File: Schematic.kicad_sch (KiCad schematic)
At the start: 73 parts, among them J1 Screw_Terminal_01x04, J20 T44007, J21 T44007, Q1 HY1707, Q20 2N2222, Q21 PMOS, U1 UC3845, U20 SFH618A-5, U21 TL431LP, U23 TCMT1108, U24 UC3843_SOIC8, U26 TL432DBZ

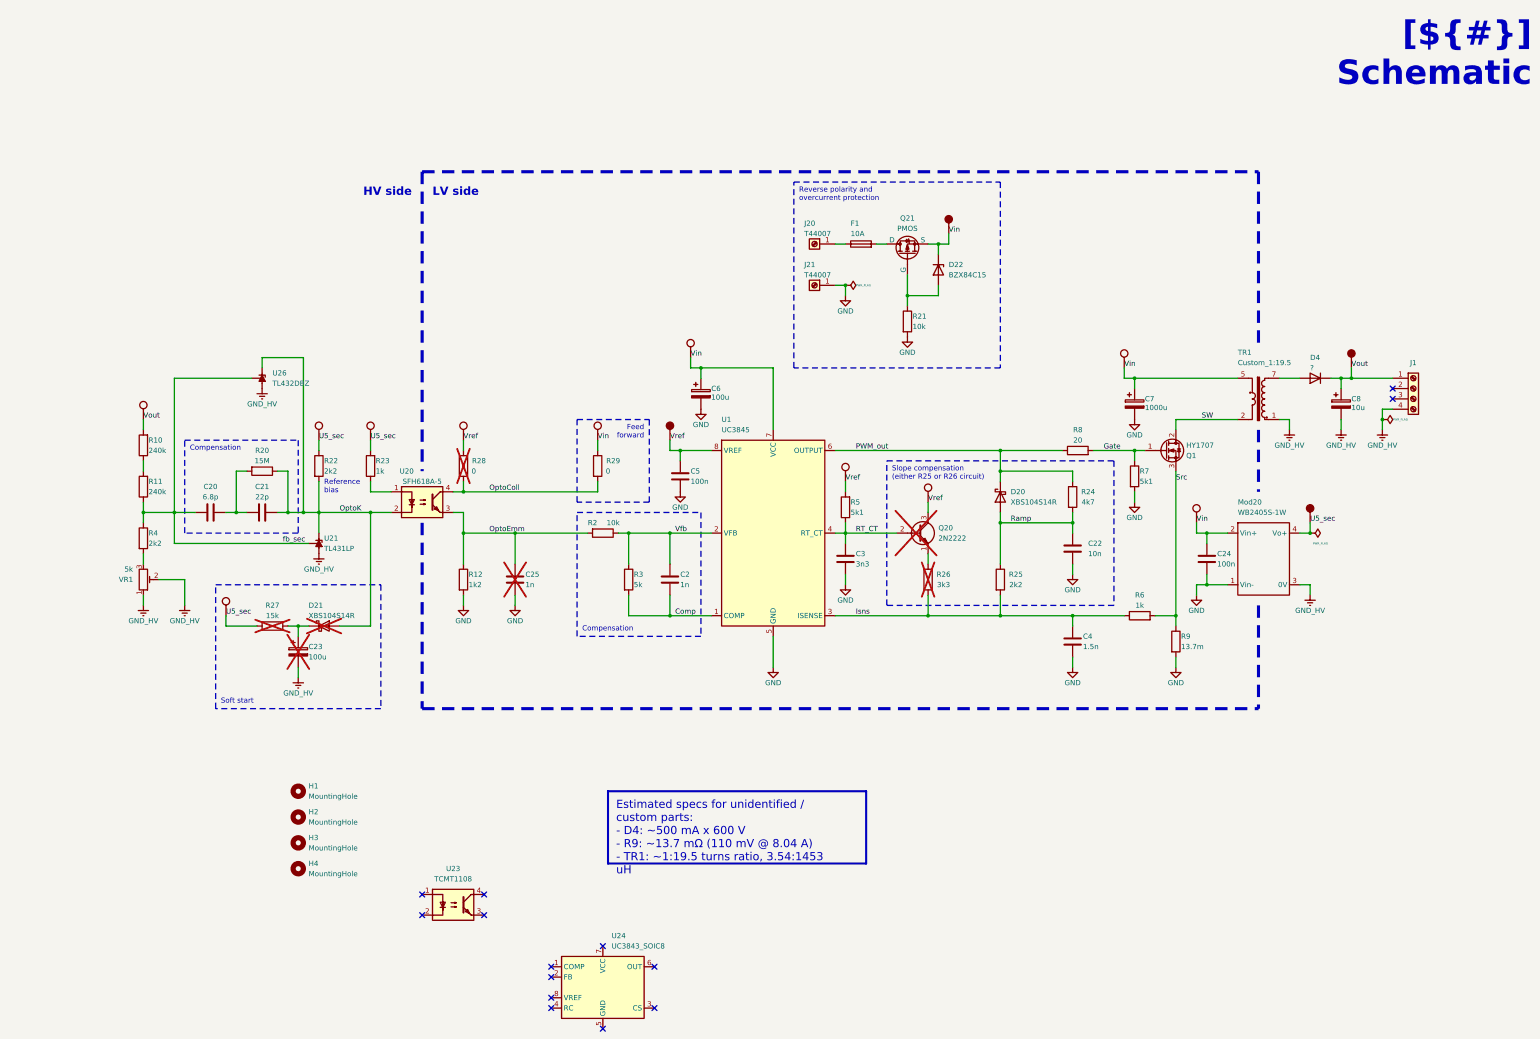
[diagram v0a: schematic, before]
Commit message: Several footprint updates
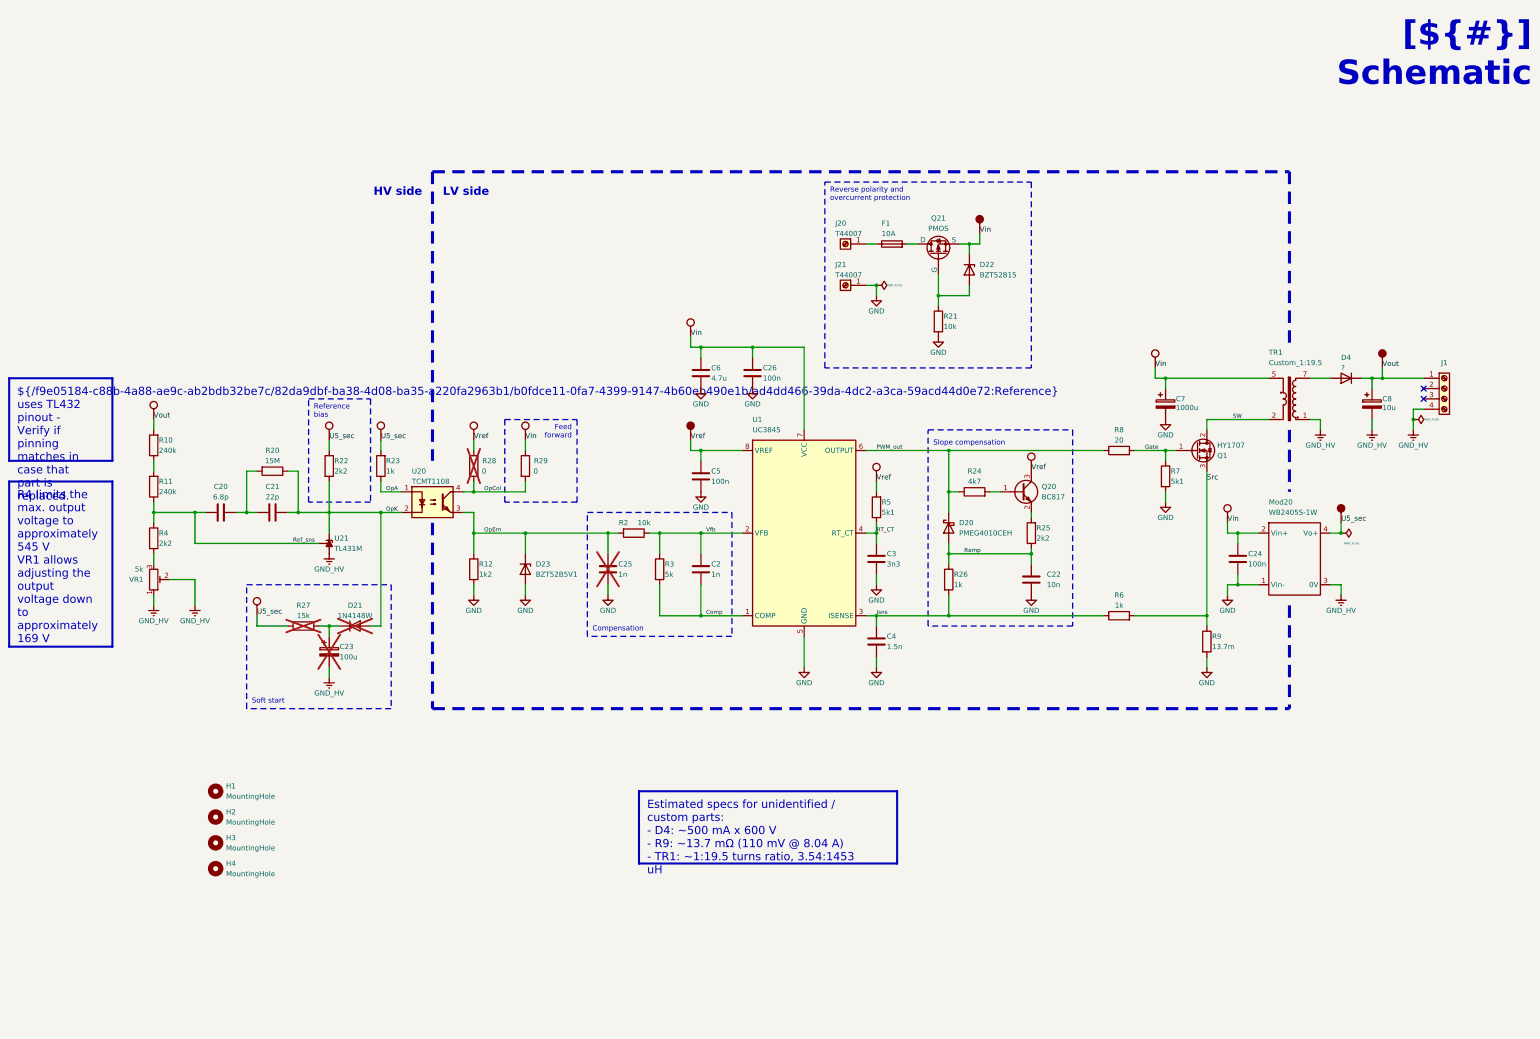
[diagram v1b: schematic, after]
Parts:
- removed C6: 100u, Capacitor_THT:C_Radial_D8.0mm_H11.5mm_P3.50mm, symbol Device:C_Polarized
- removed Q20: 2N2222, Package_TO_SOT_THT:TO-92L_Inline_Wide, symbol Transistor_BJT:2N3904
- removed U20: SFH618A-5, Package_DIP:DIP-4_W7.62mm, symbol Isolator:SFH617A-1
- removed U21: TL431LP, Package_TO_SOT_THT:TO-92L_Inline_Wide, symbol Reference_Voltage:TL431LP
- removed U24: UC3843_SOIC8, Package_SO:SOIC-8_3.9x4.9mm_P1.27mm, symbol Regulator_Controller:UC3843_SOIC8
- added C26: 100n, Capacitor_SMD:C_0603_1608Metric_Pad1.08x0.95mm_HandSolder, symbol Device:C
- added C6: 4.7u, Capacitor_SMD:C_0805_2012Metric_Pad1.18x1.45mm_HandSolder, symbol Device:C
- added D23: BZT52B5V1, Diode_SMD:D_SOD-123, symbol Device:D_Zener
- added Q20: BC817, Package_TO_SOT_SMD:SOT-23, symbol Transistor_BJT:BC817
- D20: value XBS104S14R -> PMEG4010CEH; symbol Device:D_Schottky -> Diode:PMEG4010CEH
- D21: value XBS104S14R -> 1N4148W; footprint Diode_SMD:D_SOD-123F -> Diode_SMD:D_SOD-123; symbol Device:D_Schottky -> Diode:1N4148W
- D22: value BZX84C15 -> BZT52B15; footprint Package_TO_SOT_SMD:SOT-23 -> Diode_SMD:D_SOD-123; symbol Diode:BZX84Cxx -> Diode:BZT52Bxx
- F1: footprint Fuse:Fuseholder_Clip-5x20mm_Eaton_1A5601-01_Inline_P20.80x6.76mm_D1.70mm_Horizontal -> Fuse:Fuseholder_Clip-5x20mm_Littelfuse_520_Inline_P20.50x5.80mm_D1.30mm_Horizontal
- R26: value 3k3 -> 1k; now fitted
- U1: footprint Package_DIP:DIP-8_W7.62mm -> Package_SO:JEITA_SOIC-8_3.9x4.9mm_P1.27mm
- U21: renamed from U26; value TL432DBZ -> TL431M; Link (none) -> https://www.lcsc.com/product-detail/C48947167.html; MPN (none) -> FOSAN TL431M-0.3%-6AF
- renumbered U23 to U20
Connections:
- net OptoColl is gone; now on net OpCol: R28.2, R29.2
- net OptoEmm is gone; now on net OpEm: C25.1, R12.1, R2.2
- net OptoK is gone; now on net OpK: C21.2, D21.2 (A), R20.1, R22.2, U21.2 (K)
- net GND: now also C26.2, C6.2, D23.2 (A)
- net Isns: no longer R25.2
- net Ramp: now also R26.1; no longer R24.2
- net Vin: now also D22.1 (K), C26.1, C6.1; no longer D22.3 (K)
- net Vref: now also Q20.3 (C)
- net at Q21.2 (G), R21.1: now also D22.2 (A); no longer D22.1 (A)
- net OpA: now reaches U20.1
- net OpA: now also R23.1
- net OpK: now reaches U20.2
- net OpEm: now reaches U20.3
- net OpEm: now also D23.1 (K)
- net OpCol: now reaches U20.4
- net fb_sec renamed Ref_sns
- new net: Q20.1 (B), R24.2
- new net: Q20.2 (E), R25.2
- no-connect marks 14 -> 2
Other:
- note added: "Slope compensation"
- note removed: "Slope compensation (either R25 or R26 circuit)"
- moved on the sheet: C2, C20, C21, C22, C23, C24, C25, C3, C4, C5, C7, C8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

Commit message: Layout started
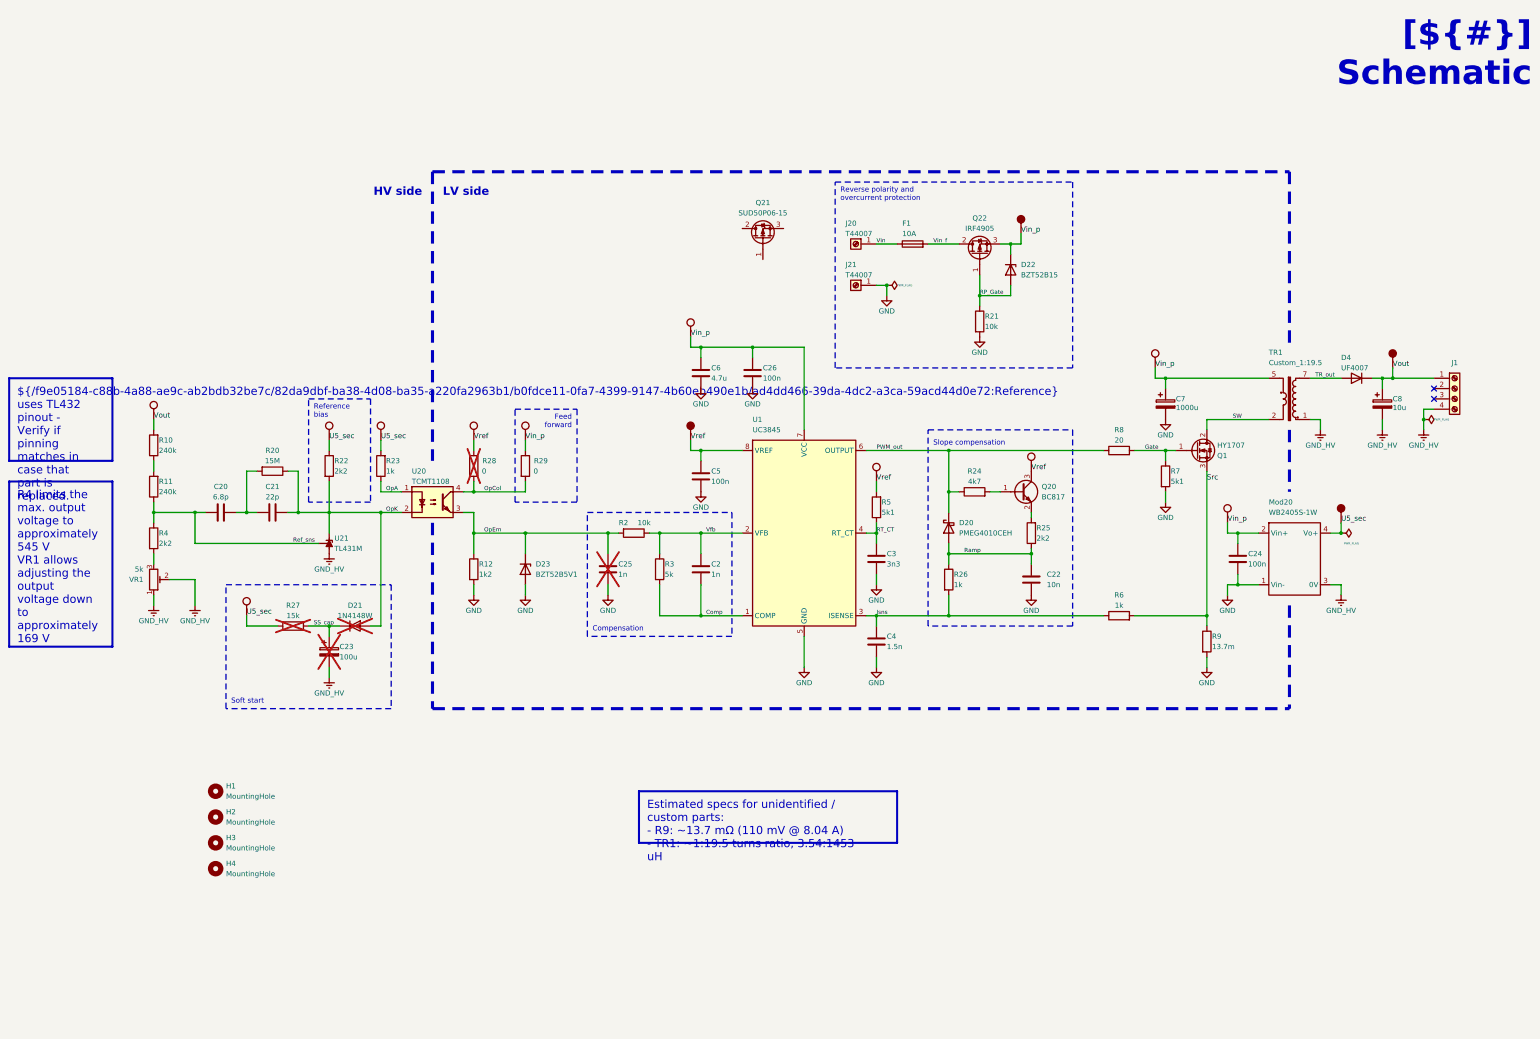
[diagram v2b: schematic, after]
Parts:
- added Q22: IRF4905, Package_TO_SOT_THT:TO-220-3_Vertical, symbol Transistor_FET:IRF4905
- D4: value ? -> UF4007
- Q21: value PMOS -> SUD50P06-15; footprint (none) -> Package_TO_SOT_SMD:TO-252-2; symbol Simulation_SPICE:PMOS -> Transistor_FET:SUD50P06-15
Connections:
- net Vin: now also F1.1, J20.1 (Pin_1); no longer C24.1, C26.1, C6.1, C7.1, D22.1 (K), Mod20.2 (Vin+), P21.1, P23.1, P24.1, P25.1, P26.1, Q21.3 (S), R29.1, TR1.5, U1.7 (VCC)
- net SS_cap: now reaches C23.1, D21.1 (K), R27.1
- net RP_Gate: now reaches D22.2 (A), R21.1
- net RP_Gate: now also Q22.1 (G); no longer Q21.2 (G)
- net TR_out: now reaches D4.2 (A), TR1.7
- net at Q21.1 (G): no longer F1.2
- new net Vin_f: F1.2, Q22.2 (D)
- new net Vin_p: C24.1, C26.1, C6.1, C7.1, D22.1 (K), Mod20.2 (Vin+), P21.1, P23.1, P24.1, P25.1, P26.1, Q22.3 (S), R29.1, TR1.5, U1.7 (VCC)
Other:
- moved on the sheet: C8, D22, D4, F1, J1, J20, J21, Q21, R21, R27
